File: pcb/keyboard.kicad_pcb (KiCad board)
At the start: 2 copper layers, 349.7 x 114.3 mm, 102 parts, among them SW1 SW_PUSH, U1 ProMicro

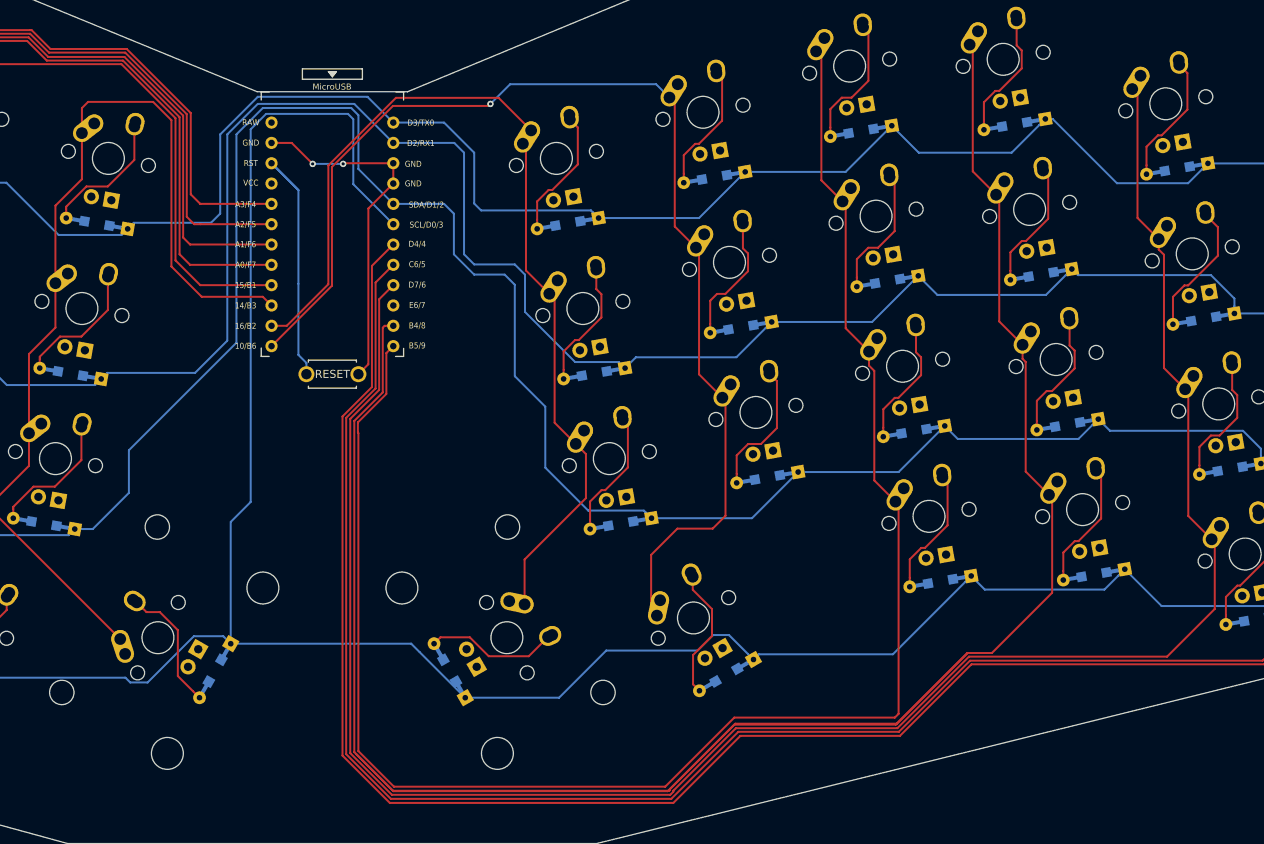
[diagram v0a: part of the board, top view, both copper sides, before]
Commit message: clean up routes
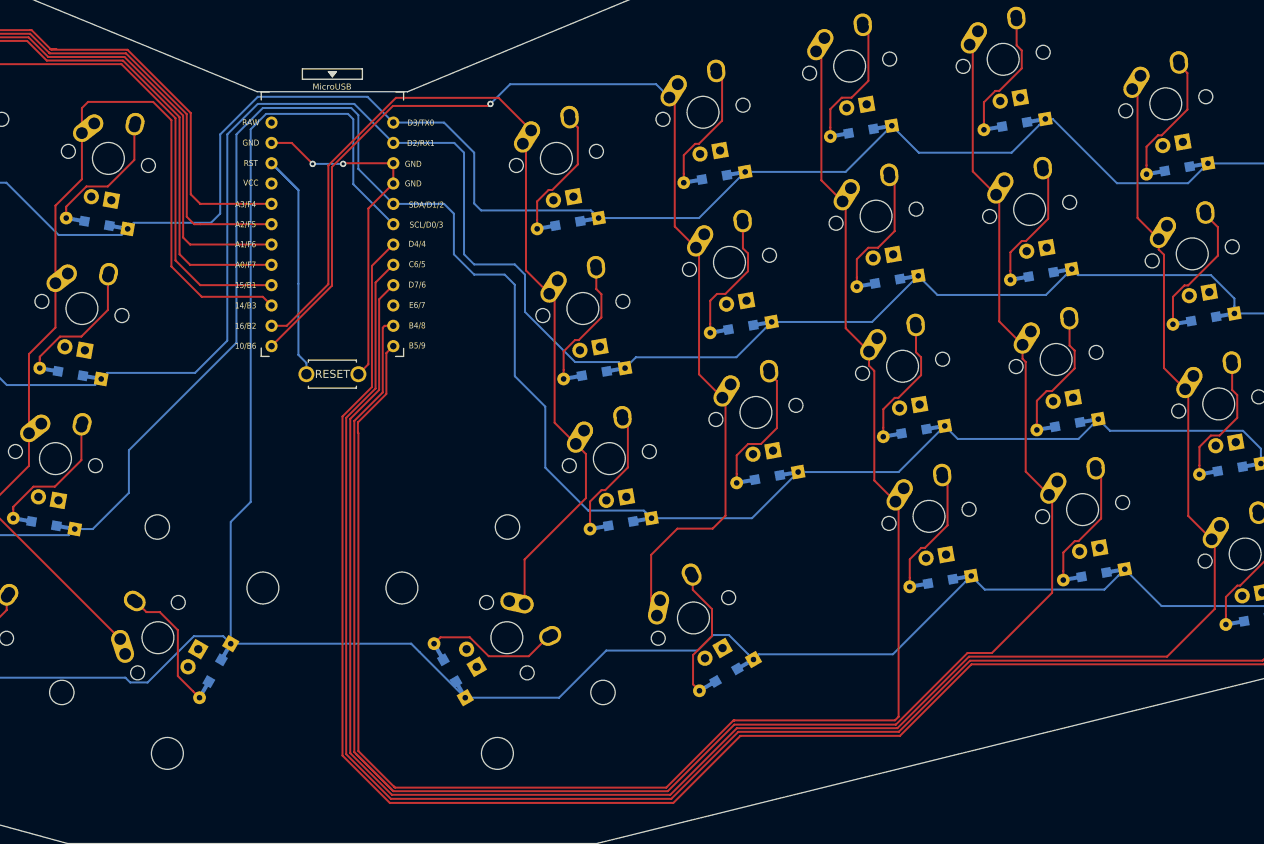
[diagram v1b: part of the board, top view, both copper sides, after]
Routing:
- net col9: track 313.8 -> 234.8 mm
- net col0: track 213.8 -> 214.6 mm
